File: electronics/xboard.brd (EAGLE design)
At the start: 78.5 x 78.5 mm, 37 parts

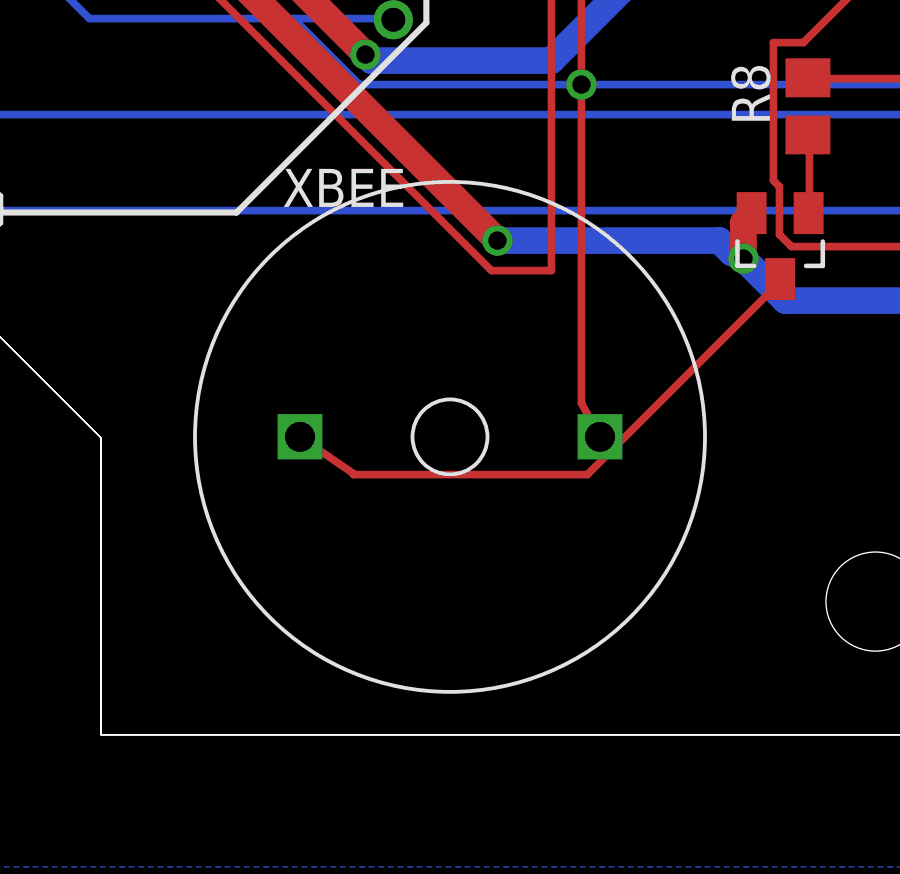
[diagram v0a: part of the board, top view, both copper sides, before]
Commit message: XBoard
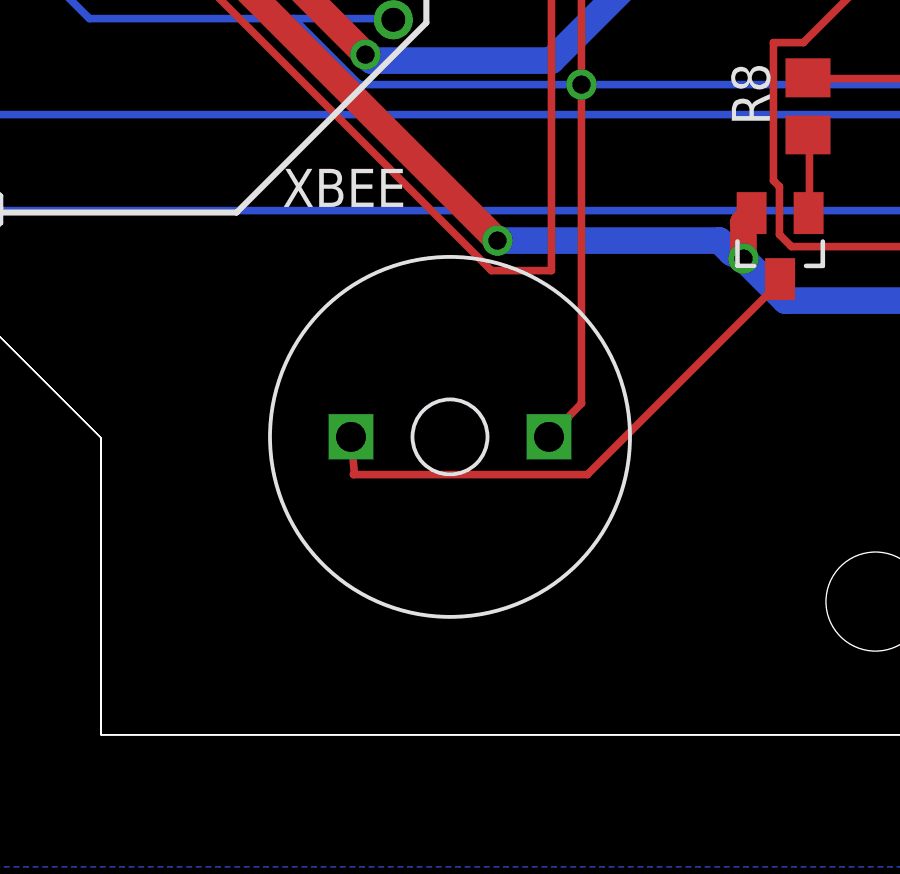
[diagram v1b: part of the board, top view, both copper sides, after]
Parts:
- BUZZER: value BUZZER10MM -> BUZZER66; device rhoban:BUZZER10 -> rhoban:BUZZER66
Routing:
- net N$5: track 19.2 -> 18.3 mm
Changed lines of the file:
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@@
 <element name="U$12" library="rhoban" package="SOT-23" value="NPN_BC817,215" x="6.4227875" y="-24.982771875" rot="R180"/>
 <element name="R8" library="rcl" package="R0805" value="470" x="7.3511" y="-20.324259375" rot="R90"/>
-<element name="BUZZER" library="rhoban" package="BUZZER10" value="BUZZER10MM" x="-4.581790625" y="-31.34356875"/>
+<element name="BUZZER" library="rhoban" package="BUZZER66" value="BUZZER66" x="-4.581790625" y="-31.34356875"/>
 <element name="CA" library="rhoban" package="C0805" value="C_EU-100NF" x="-23.6728" y="-7.112" rot="R270">
 <attribute name="FARNELL_LINK" value="http://fr.farnell.com/kemet/c0805c104j5ractu/condensateur-100nf-50v-x7r-0805/dp/1414663RL" x="-23.6728" y="-7.112" size="1.778" layer="27" rot="R270" display="off"/>
@@
 <wire x1="-0.1975375" y1="-30.227915625" x2="-0.2" y2="-30.2" width="0.254" layer="1"/>
 <wire x1="1.8" y1="-3.2" x2="1.913528125" y2="-3.1018125" width="0.254" layer="1"/>
-<wire x1="-0.1975375" y1="-30.227915625" x2="0.418209375" y2="-31.34356875" width="0.254" layer="1"/>
+<wire x1="-0.1975375" y1="-30.227915625" x2="-1.281790625" y2="-31.34356875" width="0.254" layer="1"/>
 <wire x1="15" y1="9.4" x2="18.2" y2="12.6" width="0.254" layer="1"/>
 <wire x1="15" y1="1.6" x2="15" y2="9.4" width="0.254" layer="1"/>
@@
 <wire x1="-7.765228125" y1="-32.59051875" x2="-7.8" y2="-32.6" width="0.254" layer="1"/>
 <wire x1="6.4" y1="-26.2" x2="6.4227875" y2="-26.082771875" width="0.254" layer="1"/>
-<wire x1="-7.765228125" y1="-32.59051875" x2="-9.581790625" y2="-31.34356875" width="0.254" layer="1"/>
+<wire x1="-7.765228125" y1="-32.59051875" x2="-7.881790625" y2="-31.34356875" width="0.254" layer="1"/>
 </signal>
 </signals>
